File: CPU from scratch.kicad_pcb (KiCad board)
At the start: 2 copper layers, 144.8 x 142.2 mm, 372 parts, among them Q1 2N3904, Q10 2N3904, Q11 2N3904, Q12 2N3904, Q13 2N3904, Q14 2N3904, Q15 2N3904, Q16 2N3904, Q17 2N3904, Q18 2N3904, Q19 2N3904, Q2 2N3904, Q20 2N3904, Q21 2N3904, Q3 2N3904, Q4 2N3904, Q5 2N3904, Q6 2N3904, Q7 2N3904, Q8 2N3904, Q9 2N3904

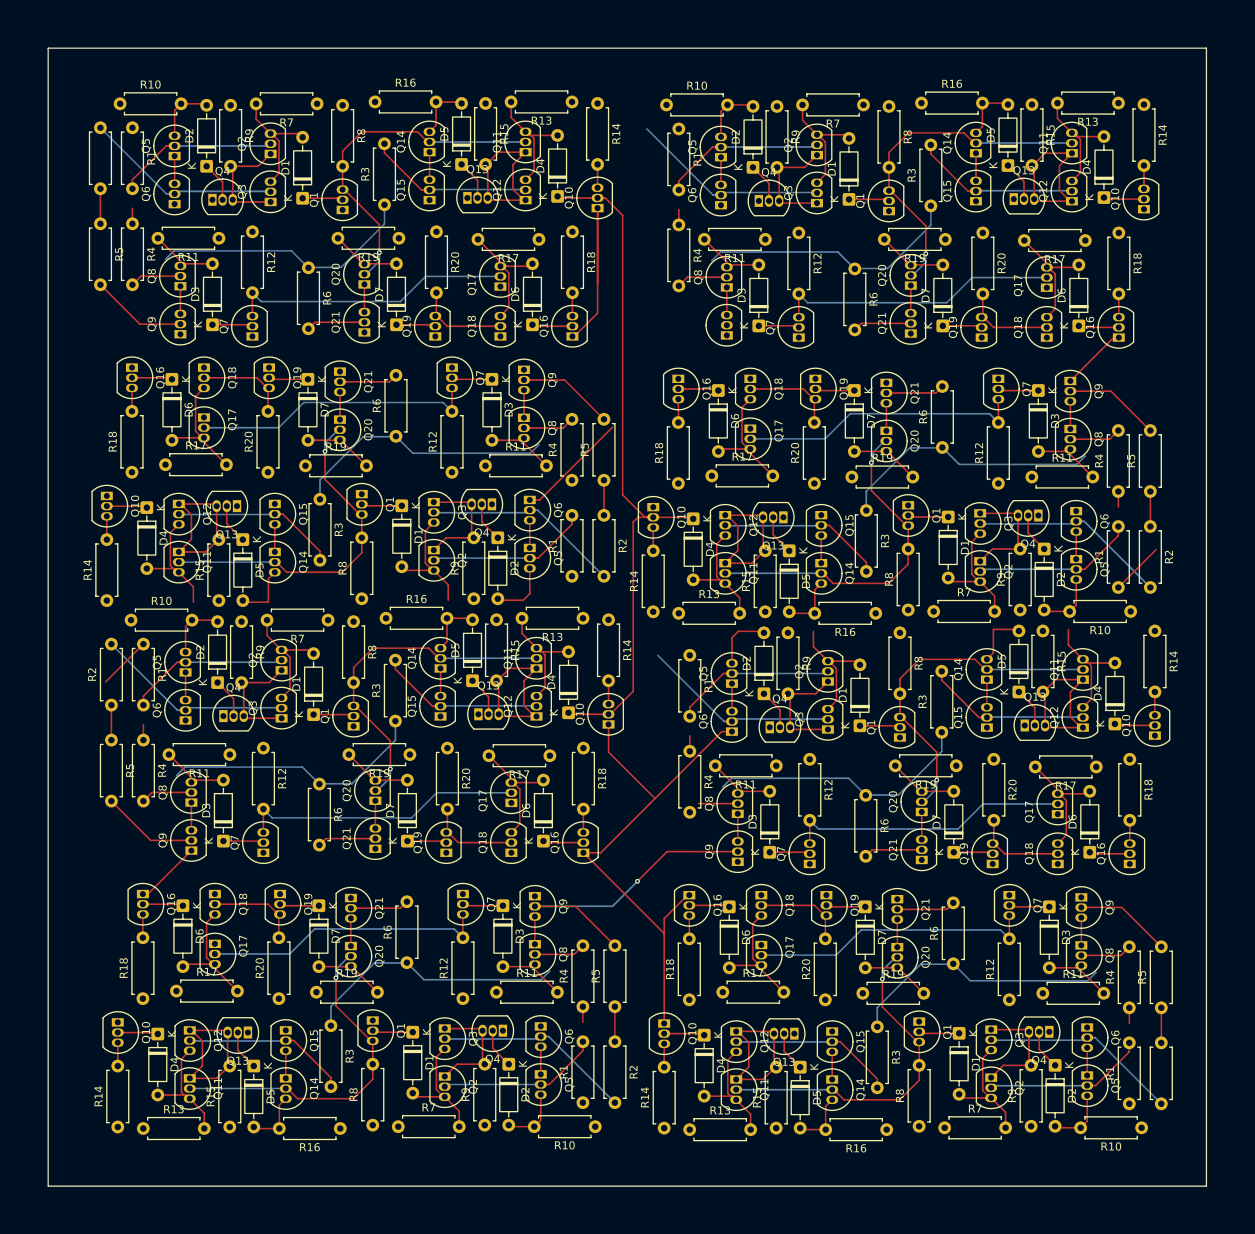
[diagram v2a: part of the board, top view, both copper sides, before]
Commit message: Update PCB
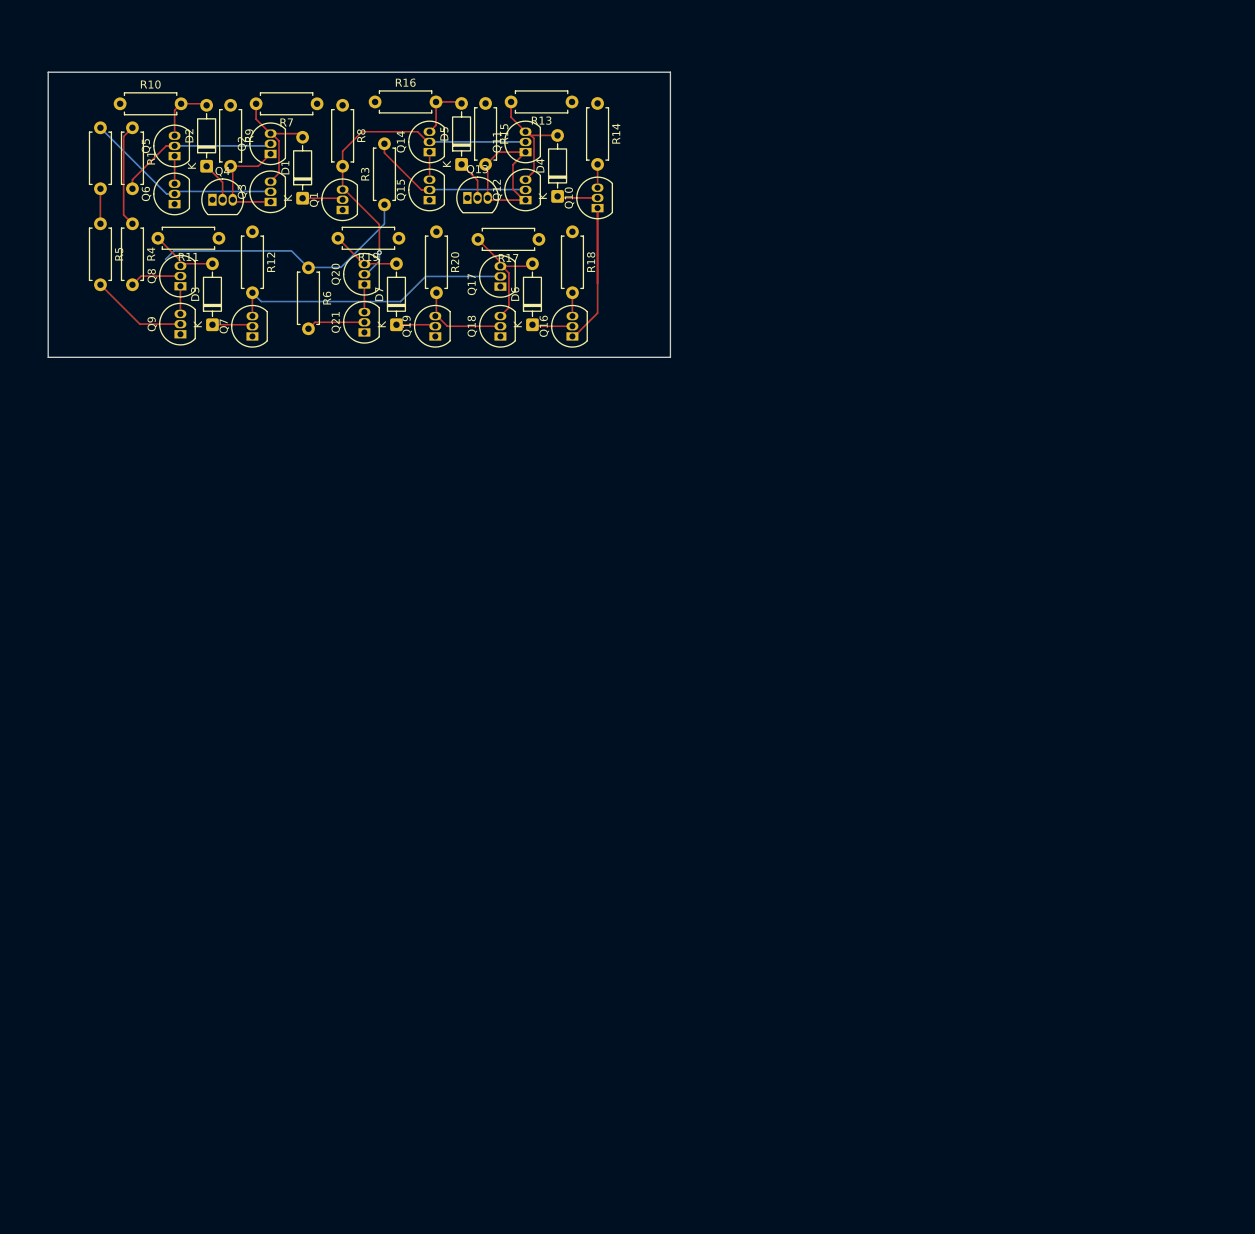
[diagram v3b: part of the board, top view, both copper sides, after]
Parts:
- removed the D1 at (136.9, 117.5)
- removed the D1 at (149.3, 157.2)
- removed the D1 at (147.9, 91.4)
- removed the D1 at (217.6, 157.3)
- removed the D1 at (203.8, 53.1)
- removed the D1 at (216.2, 92.8)
- removed the D1 at (205.2, 118.9)
- removed the D2 at (161.3, 161.2)
- removed the D2 at (228.2, 96.8)
- removed the D2 at (191.8, 49.1)
- removed the D2 at (193.2, 114.9)
- removed the D2 at (229.6, 161.3)
- removed the D2 at (124.9, 113.5)
- removed the D2 at (159.9, 95.4)
- removed the D3 at (160.6, 141.4)
- removed the D3 at (192.5, 68.9)
- removed the D3 at (193.9, 134.7)
- removed the D3 at (159.2, 75.6)
- removed the D3 at (228.9, 141.5)
- removed the D3 at (125.6, 133.3)
- removed the D3 at (227.5, 77.0)
- removed the D4 at (237.1, 118.7)
- removed the D4 at (116.0, 91.6)
- removed the D4 at (168.8, 117.3)
- removed the D4 at (185.7, 157.6)
- removed the D4 at (117.4, 157.4)
- removed the D4 at (235.7, 52.9)
- removed the D4 at (184.3, 93.0)
- removed the D5 at (129.4, 161.4)
- removed the D5 at (223.7, 48.9)
- removed the D5 at (196.3, 97.0)
- removed the D5 at (156.8, 113.3)
- removed the D5 at (225.1, 114.7)
- removed the D5 at (128.0, 95.6)
- removed the D5 at (197.7, 161.6)
- removed the D6 at (188.9, 141.5)
- removed the D6 at (120.6, 141.4)
- removed the D6 at (165.6, 133.3)
- removed the D6 at (233.9, 134.7)
- removed the D6 at (187.5, 77.0)
- removed the D6 at (119.2, 75.6)
- removed the D6 at (232.5, 68.9)
- removed the D7 at (137.6, 141.4)
- removed the D7 at (204.5, 77.0)
- removed the D7 at (216.9, 134.7)
- removed the D7 at (136.2, 75.6)
- removed the D7 at (215.5, 68.9)
- removed the D7 at (205.9, 141.5)
- removed the D7 at (148.6, 133.3)
- removed the Q1 at (144.3, 155.7)
- removed the Q1 at (208.8, 54.6)
- removed the Q1 at (211.2, 91.3)
- removed the Q1 at (141.9, 119.0)
- removed the Q1 at (210.2, 120.4)
- removed the Q1 at (142.9, 89.9)
- removed the Q1 at (212.6, 155.9)
- removed the Q10 at (242.1, 120.1)
- removed the Q10 at (179.3, 91.6)
- removed the Q10 at (111.0, 90.2)
- removed the Q10 at (112.4, 156.0)
- removed the Q10 at (180.7, 156.1)
- removed the Q10 at (240.7, 54.3)
- removed the Q10 at (173.8, 118.7)
- removed the Q11 at (189.7, 163.1)
- removed the Q11 at (188.3, 98.6)
- removed the Q11 at (121.4, 163.0)
- removed the Q11 at (164.8, 111.7)
- removed the Q11 at (231.7, 47.3)
- removed the Q11 at (120.0, 97.2)
- removed the Q11 at (233.1, 113.1)
- removed the Q12 at (120.0, 91.2)
- removed the Q12 at (164.8, 117.7)
- removed the Q12 at (121.4, 157.0)
- removed the Q12 at (188.3, 92.6)
- removed the Q12 at (231.7, 53.3)
- removed the Q12 at (233.1, 119.1)
- removed the Q12 at (189.7, 157.1)
- removed the Q13 at (225.8, 118.9)
- removed the Q13 at (224.4, 53.1)
- removed the Q13 at (157.5, 117.5)
- removed the Q13 at (197.0, 157.4)
- removed the Q13 at (195.6, 92.8)
- removed the Q13 at (128.7, 157.2)
- removed the Q13 at (127.3, 91.4)
- removed the Q14 at (132.0, 97.2)
- removed the Q14 at (221.1, 113.1)
- removed the Q14 at (133.4, 163.0)
- removed the Q14 at (152.8, 111.7)
- removed the Q14 at (200.3, 98.6)
- removed the Q14 at (201.7, 163.1)
- removed the Q14 at (219.7, 47.3)
- removed the Q15 at (219.7, 53.3)
- removed the Q15 at (133.4, 157.0)
- removed the Q15 at (132.0, 91.2)
- removed the Q15 at (152.8, 117.7)
- removed the Q15 at (221.1, 119.1)
- removed the Q15 at (201.7, 157.1)
- removed the Q15 at (200.3, 92.6)
- removed the Q16 at (183.9, 140.1)
- removed the Q16 at (237.5, 70.4)
- removed the Q16 at (170.6, 134.8)
- removed the Q16 at (115.6, 139.9)
- removed the Q16 at (238.9, 136.2)
- removed the Q16 at (114.2, 74.1)
- removed the Q16 at (182.5, 75.5)
- removed the Q17 at (123.2, 80.4)
- removed the Q17 at (229.9, 129.9)
- removed the Q17 at (161.6, 128.5)
- removed the Q17 at (191.5, 81.8)
- removed the Q17 at (192.9, 146.3)
- removed the Q17 at (228.5, 64.1)
- removed the Q17 at (124.6, 146.2)
- removed the Q18 at (229.9, 136.2)
- removed the Q18 at (191.5, 75.5)
- removed the Q18 at (192.9, 140.1)
- removed the Q18 at (123.2, 74.1)
- removed the Q18 at (161.6, 134.8)
- removed the Q18 at (228.5, 70.4)
- removed the Q18 at (124.6, 139.9)
- removed the Q19 at (220.4, 70.4)
- removed the Q19 at (153.5, 134.8)
- removed the Q19 at (132.7, 139.9)
- removed the Q19 at (221.8, 136.2)
- removed the Q19 at (201.0, 140.1)
- removed the Q19 at (131.3, 74.1)
- removed the Q19 at (199.6, 75.5)
- removed the Q2 at (220.2, 98.3)
- removed the Q2 at (199.8, 47.6)
- removed the Q2 at (201.2, 113.4)
- removed the Q2 at (221.6, 162.9)
- removed the Q2 at (153.3, 162.7)
- removed the Q2 at (151.9, 96.9)
- removed the Q2 at (132.9, 112.0)
- removed the Q20 at (211.5, 63.9)
- removed the Q20 at (144.6, 128.3)
- removed the Q20 at (141.6, 146.4)
- removed the Q20 at (208.5, 82.0)
- removed the Q20 at (140.2, 80.6)
- removed the Q20 at (212.9, 129.7)
- removed the Q20 at (209.9, 146.6)
- removed the Q21 at (209.9, 140.6)
- removed the Q21 at (141.6, 140.4)
- removed the Q21 at (140.2, 74.6)
- removed the Q21 at (212.9, 135.7)
- removed the Q21 at (211.5, 69.9)
- removed the Q21 at (208.5, 76.0)
- removed the Q21 at (144.6, 134.3)
- removed the Q3 at (201.2, 119.4)
- removed the Q3 at (153.3, 156.7)
- removed the Q3 at (151.9, 90.9)
- removed the Q3 at (132.9, 118.0)
- removed the Q3 at (221.6, 156.9)
- removed the Q3 at (199.8, 53.6)
- removed the Q3 at (220.2, 92.3)
- removed the Q4 at (228.9, 157.2)
- removed the Q4 at (193.9, 119.1)
- removed the Q4 at (125.6, 117.7)
- removed the Q4 at (159.2, 91.2)
- removed the Q4 at (160.6, 157.0)
- removed the Q4 at (227.5, 92.6)
- removed the Q4 at (192.5, 53.3)
- removed the Q5 at (187.8, 47.8)
- removed the Q5 at (165.3, 162.5)
- removed the Q5 at (163.9, 96.7)
- removed the Q5 at (189.2, 113.6)
- removed the Q5 at (233.6, 162.6)
- removed the Q5 at (232.2, 98.1)
- removed the Q5 at (120.9, 112.2)
- removed the Q6 at (233.6, 156.6)
- removed the Q6 at (187.8, 53.8)
- removed the Q6 at (163.9, 90.7)
- removed the Q6 at (165.3, 156.5)
- removed the Q6 at (232.2, 92.1)
- removed the Q6 at (189.2, 119.6)
- removed the Q6 at (120.9, 118.2)
- removed the Q7 at (198.9, 136.2)
- removed the Q7 at (155.6, 139.9)
- removed the Q7 at (222.5, 75.5)
- removed the Q7 at (154.2, 74.1)
- removed the Q7 at (130.6, 134.8)
- removed the Q7 at (197.5, 70.4)
- removed the Q7 at (223.9, 140.1)
- removed the Q8 at (232.9, 146.3)
- removed the Q8 at (189.9, 129.9)
- removed the Q8 at (188.5, 64.1)
- removed the Q8 at (121.6, 128.5)
- removed the Q8 at (164.6, 146.2)
- removed the Q8 at (163.2, 80.4)
- removed the Q8 at (231.5, 81.8)
- removed the Q9 at (232.9, 140.3)
- removed the Q9 at (189.9, 135.9)
- removed the Q9 at (231.5, 75.8)
- removed the Q9 at (121.6, 134.5)
- removed the Q9 at (188.5, 70.1)
- removed the Q9 at (163.2, 74.4)
- removed the Q9 at (164.6, 140.2)
- removed the R1 at (182.5, 44.3)
- removed the R1 at (169.2, 100.2)
- removed the R1 at (183.9, 110.1)
- removed the R1 at (237.5, 101.6)
- removed the R1 at (170.6, 166.0)
- removed the R1 at (238.9, 166.2)
- removed the R1 at (115.6, 108.7)
- removed the R10 at (239.0, 104.6)
- removed the R10 at (181.0, 41.3)
- removed the R10 at (114.1, 105.7)
- removed the R10 at (172.1, 169.0)
- removed the R10 at (240.4, 169.2)
- removed the R11 at (159.7, 152.2)
- removed the R11 at (228.0, 152.3)
- removed the R11 at (193.4, 58.1)
- removed the R11 at (158.4, 86.4)
- removed the R11 at (126.4, 122.5)
- removed the R11 at (226.7, 87.8)
- removed the R11 at (194.7, 123.9)
- removed the R12 at (197.5, 57.3)
- removed the R12 at (154.2, 87.2)
- removed the R12 at (130.6, 121.7)
- removed the R12 at (222.5, 88.6)
- removed the R12 at (155.6, 153.0)
- removed the R12 at (223.9, 153.2)
- removed the R12 at (198.9, 123.1)
- removed the R13 at (183.9, 169.4)
- removed the R13 at (115.6, 169.2)
- removed the R13 at (237.5, 41.1)
- removed the R13 at (170.6, 105.5)
- removed the R13 at (182.5, 104.8)
- removed the R14 at (240.7, 41.3)
- removed the R14 at (242.1, 107.1)
- removed the R14 at (111.0, 103.3)
- removed the R14 at (173.8, 105.7)
- removed the R14 at (112.4, 169.1)
- removed the R14 at (179.3, 104.7)
- removed the R14 at (180.7, 169.2)
- removed the R15 at (125.0, 103.3)
- removed the R15 at (159.8, 105.7)
- removed the R15 at (226.7, 41.3)
- removed the R15 at (228.1, 107.1)
- removed the R15 at (126.4, 169.1)
- removed the R15 at (194.7, 169.2)
- removed the R15 at (193.3, 104.7)
- removed the R16 at (208.5, 169.4)
- removed the R16 at (140.2, 169.2)
- removed the R16 at (145.9, 105.5)
- removed the R16 at (207.2, 104.8)
- removed the R16 at (212.9, 41.1)
- removed the R17 at (118.4, 86.3)
- removed the R17 at (233.4, 58.2)
- removed the R17 at (166.4, 122.6)
- removed the R17 at (119.7, 152.1)
- removed the R17 at (188.0, 152.2)
- removed the R17 at (234.7, 124.0)
- removed the R17 at (186.7, 87.7)
- removed the R18 at (114.2, 87.2)
- removed the R18 at (237.5, 57.3)
- removed the R18 at (170.6, 121.7)
- removed the R18 at (182.5, 88.6)
- removed the R18 at (115.6, 153.0)
- removed the R18 at (238.9, 123.1)
- removed the R18 at (183.9, 153.2)
- removed the R19 at (204.2, 87.8)
- removed the R19 at (215.9, 58.1)
- removed the R19 at (137.2, 152.2)
- removed the R19 at (148.9, 122.5)
- removed the R19 at (217.2, 123.9)
- removed the R19 at (135.9, 86.4)
- removed the R19 at (205.5, 152.3)
- removed the R2 at (241.5, 94.0)
- removed the R2 at (173.2, 92.6)
- removed the R2 at (174.6, 158.4)
- removed the R2 at (111.6, 116.3)
- removed the R2 at (242.9, 158.5)
- removed the R20 at (199.5, 88.6)
- removed the R20 at (221.9, 123.1)
- removed the R20 at (153.6, 121.7)
- removed the R20 at (132.6, 153.0)
- removed the R20 at (131.2, 87.2)
- removed the R20 at (200.9, 153.2)
- removed the R20 at (220.5, 57.3)
- removed the R3 at (207.4, 156.5)
- removed the R3 at (206.0, 92.0)
- removed the R3 at (215.4, 119.7)
- removed the R3 at (214.0, 53.9)
- removed the R3 at (147.1, 118.3)
- removed the R3 at (137.7, 90.6)
- removed the R3 at (139.1, 156.4)
- removed the R4 at (237.5, 89.6)
- removed the R4 at (183.9, 122.1)
- removed the R4 at (170.6, 154.0)
- removed the R4 at (238.9, 154.2)
- removed the R4 at (169.2, 88.2)
- removed the R4 at (182.5, 56.3)
- removed the R4 at (115.6, 120.7)
- removed the R5 at (174.6, 154.0)
- removed the R5 at (242.9, 154.2)
- removed the R5 at (111.6, 120.7)
- removed the R5 at (241.5, 89.6)
- removed the R5 at (173.2, 88.2)
- removed the R6 at (148.6, 148.5)
- removed the R6 at (215.5, 84.1)
- removed the R6 at (137.6, 126.2)
- removed the R6 at (205.9, 127.6)
- removed the R6 at (204.5, 61.8)
- removed the R6 at (147.2, 82.7)
- removed the R6 at (216.9, 148.7)
- removed the R7 at (215.8, 169.2)
- removed the R7 at (214.4, 104.6)
- removed the R7 at (205.6, 41.3)
- removed the R7 at (138.7, 105.7)
- removed the R7 at (147.5, 169.0)
- removed the R8 at (211.2, 104.4)
- removed the R8 at (210.2, 107.3)
- removed the R8 at (208.8, 41.5)
- removed the R8 at (212.6, 169.0)
- removed the R8 at (142.9, 103.0)
- removed the R8 at (141.9, 105.9)
- removed the R8 at (144.3, 168.8)
- removed the R9 at (158.3, 168.8)
- removed the R9 at (225.2, 104.4)
- removed the R9 at (194.8, 41.5)
- removed the R9 at (127.9, 105.9)
- removed the R9 at (226.6, 169.0)
- removed the R9 at (156.9, 103.0)
- removed the R9 at (196.2, 107.3)
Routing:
- net /AND2/In1: track 341.8 -> 42.7 mm, vias 8 -> 1
- net /AND1/O: track 285.4 -> 35.7 mm
- net Cin: track 266.8 -> 33.4 mm
- net /XOR1/In2: track 198.8 -> 24.8 mm
- net Net-(Q11-E): track 179.5 -> 22.4 mm
- net /XOR2/In2: track 165.9 -> 20.7 mm
- net /XOR1/In1: track 165.1 -> 20.6 mm
- net Net-(D6-A): track 127.1 -> 15.9 mm
- net Net-(D1-A): track 126.7 -> 15.8 mm
- net Net-(D4-A): track 125.4 -> 15.7 mm
- net Net-(D4-K): track 112.8 -> 5.08 mm
- net Net-(Q2-E): track 118.3 -> 14.8 mm
- net GND: track 126.3 -> 26.9 mm
- net /AND1/In2: track 100.4 -> 12.0 mm, vias 1 -> 0
- net /AND2/O: track 93.2 -> 11.6 mm
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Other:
- board size 144.8 x 142.2 mm -> 77.8 x 35.6 mm
